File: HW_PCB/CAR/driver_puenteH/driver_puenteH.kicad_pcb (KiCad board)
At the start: 2 copper layers, 33.8 x 29.5 mm, 6 parts, among them IC1 TB6612FNG, J3 Puente H, J4 Puente_H2

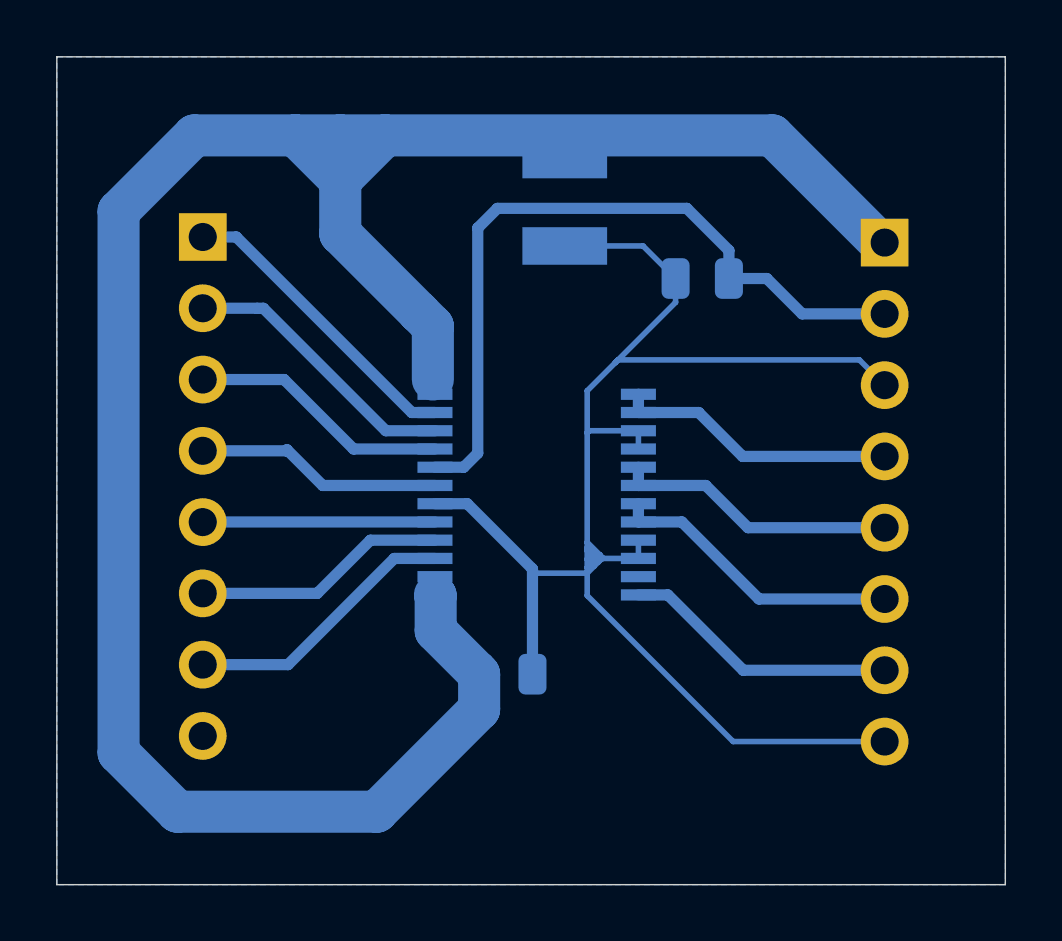
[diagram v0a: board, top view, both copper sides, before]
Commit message: Carrito pcb, 25-02-26
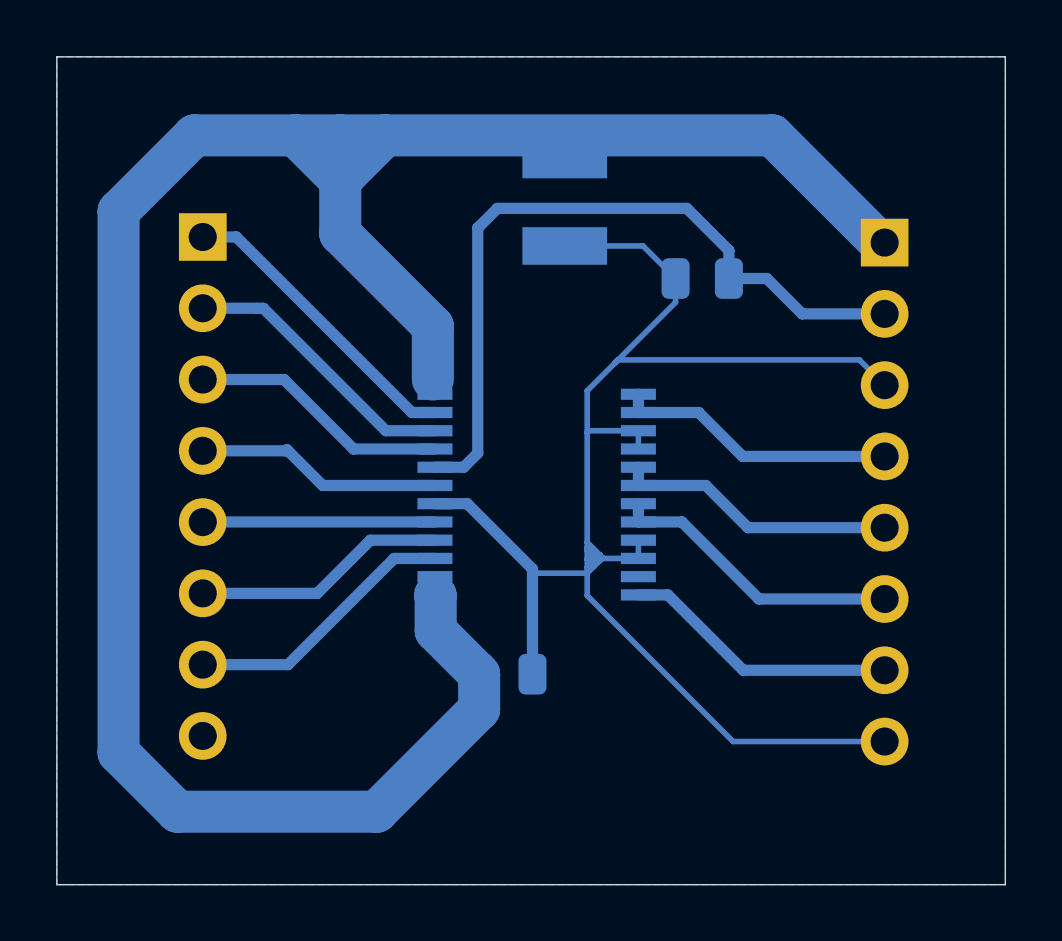
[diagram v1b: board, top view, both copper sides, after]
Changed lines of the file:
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@@
+	)
+	(segment
+		(start 133.6 69.2)
+		(end 133.6 67.3)
+		(width 1.5)
+		(layer "B.Cu")
+		(net 2)
 	)
 	(segment
@@
 	)
 	(segment
-		(start 136.4 72)
+		(start 136.9 74.4)
 		(end 136.9 72.5)
-		(width 1.5)
-		(layer "B.Cu")
-		(net 2)
-	)
-	(segment
-		(start 133.6 67.3)
-		(end 133.6 69.2)
 		(width 1.5)
 		(layer "B.Cu")
@@
 	)
 	(segment
-		(start 133.6 69.2)
-		(end 136.4 72)
-		(width 1.5)
-		(layer "B.Cu")
-		(net 2)
-	)
-	(segment
 		(start 138.55 84.9)
 		(end 137 83.35)
@@
 	(segment
 		(start 136.9 72.5)
-		(end 136.9 74.4)
+		(end 133.6 69.2)
 		(width 1.5)
 		(layer "B.Cu")

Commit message: Correción menor
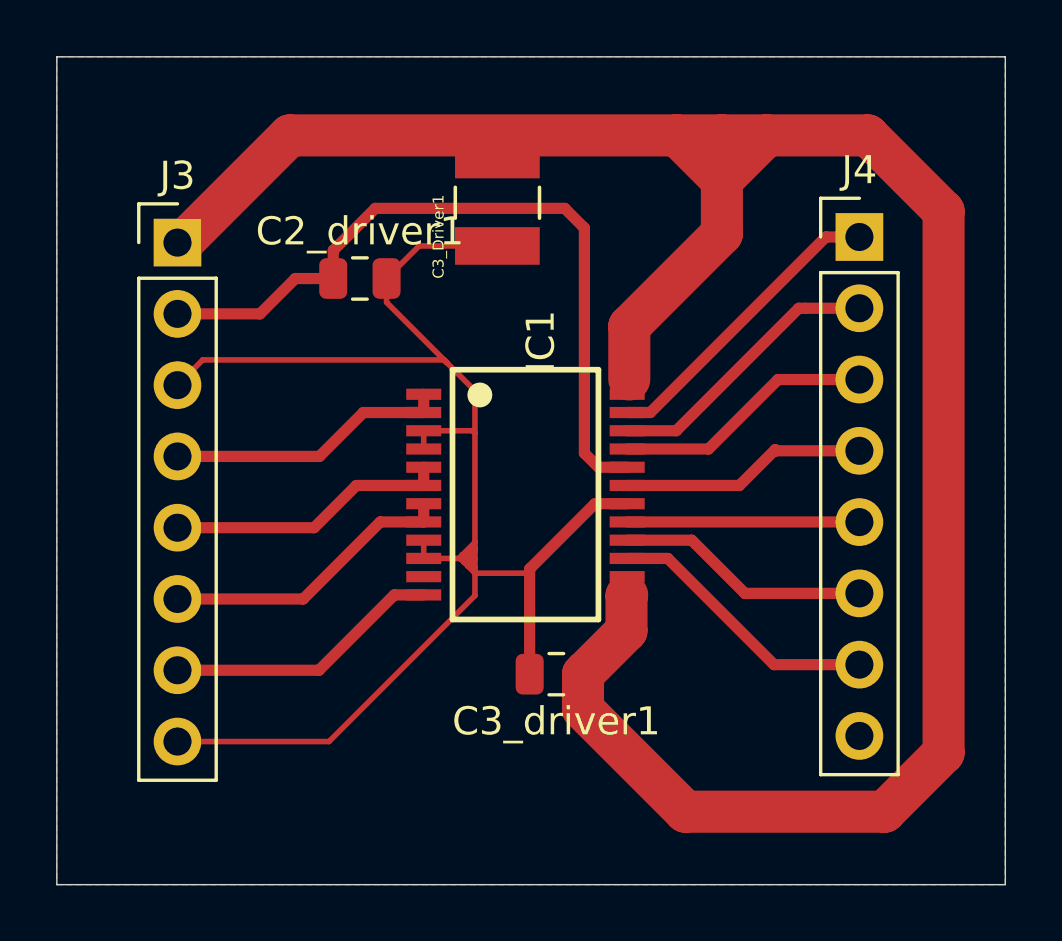
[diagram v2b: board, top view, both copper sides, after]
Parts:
- C2_driver1, C3_Driver1, C3_driver1, IC1, J3, J4: moved to F.Cu
- moved J3 25.2 mm to (127.8, 69.5), turned to 0 degrees
- moved J4 23.4 mm to (152.1, 69.3), turned to 0 degrees
- moved C2_driver1 12.2 mm to (134.3, 70.8), turned to 0 degrees
- moved C3_Driver1 2.40 mm to (139.2, 68.1)
- moved C3_driver1 1.80 mm to (141.3, 84.9), turned to 180 degrees
- moved IC1 0.40 mm to (140.2, 78.5)
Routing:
- added copper zone on F.Cu, net GND
- removed copper zone on B.Cu, net GND
